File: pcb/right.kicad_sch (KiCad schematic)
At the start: 55 parts, among them SW1 SW_PUSH, SW10 SW_PUSH, SW11 SW_PUSH, SW12 SW_PUSH, SW13 SW_PUSH, SW14 SW_PUSH, SW15 SW_PUSH, SW16 SW_PUSH, SW17 SW_PUSH, SW18 SW_PUSH, SW19 SW_PUSH, SW2 SW_PUSH, SW20 SW_PUSH, SW3 SW_PUSH, SW4 SW_PUSH, SW5 SW_PUSH, SW6 SW_PUSH, SW7 SW_PUSH, SW8 SW_PUSH, SW9 SW_PUSH, U1 xiao-ble

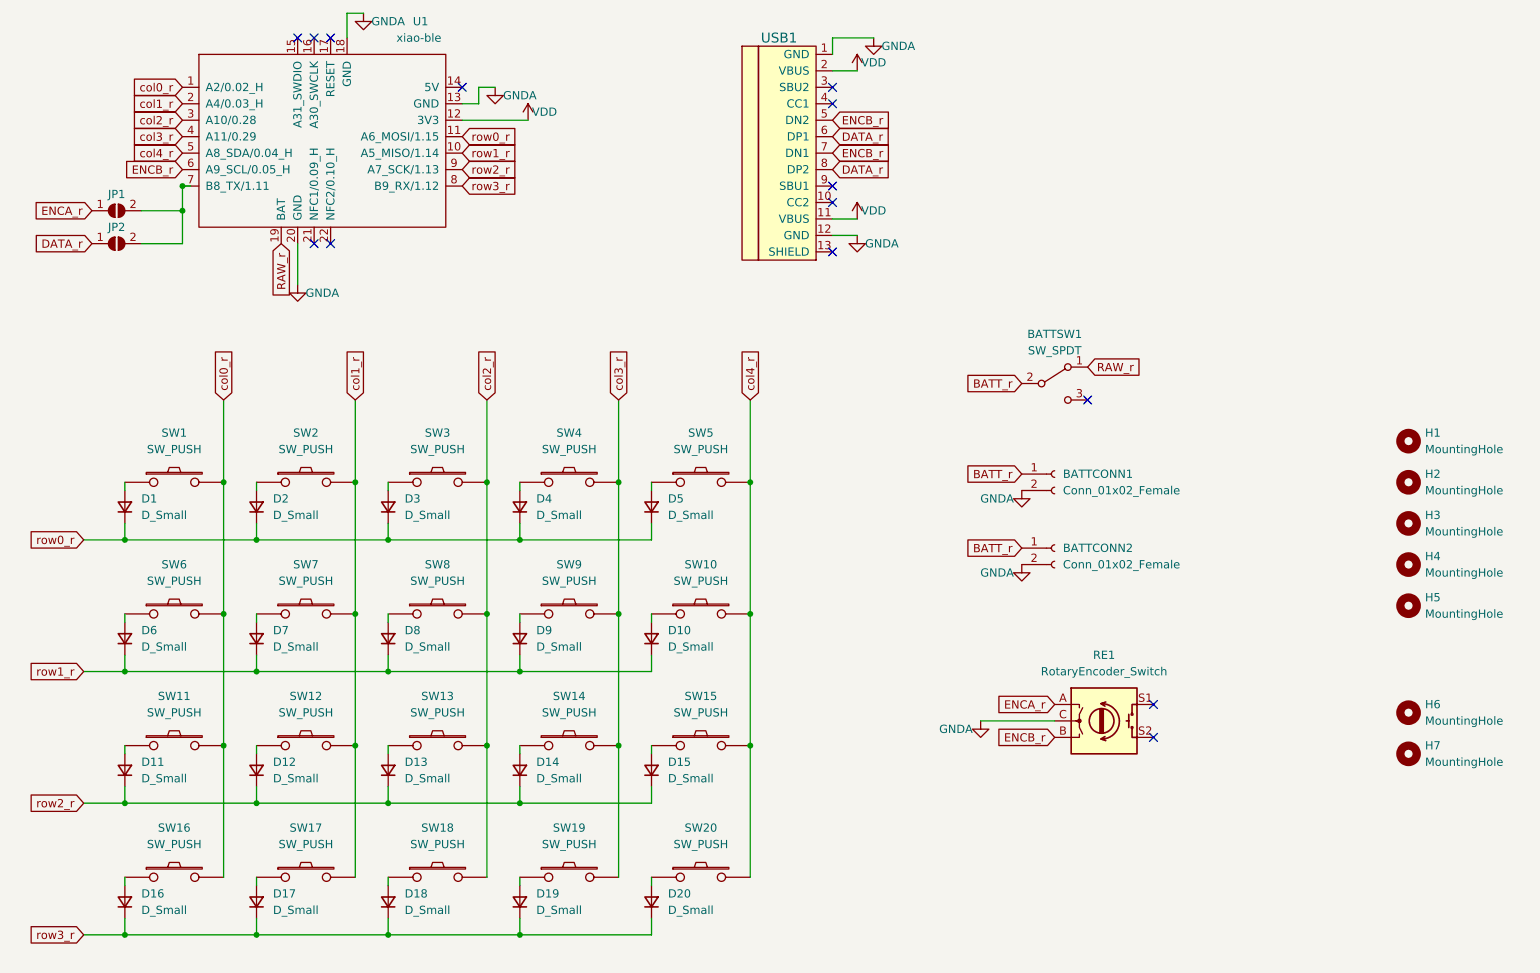
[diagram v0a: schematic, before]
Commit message: udpate pcb, remove unused files
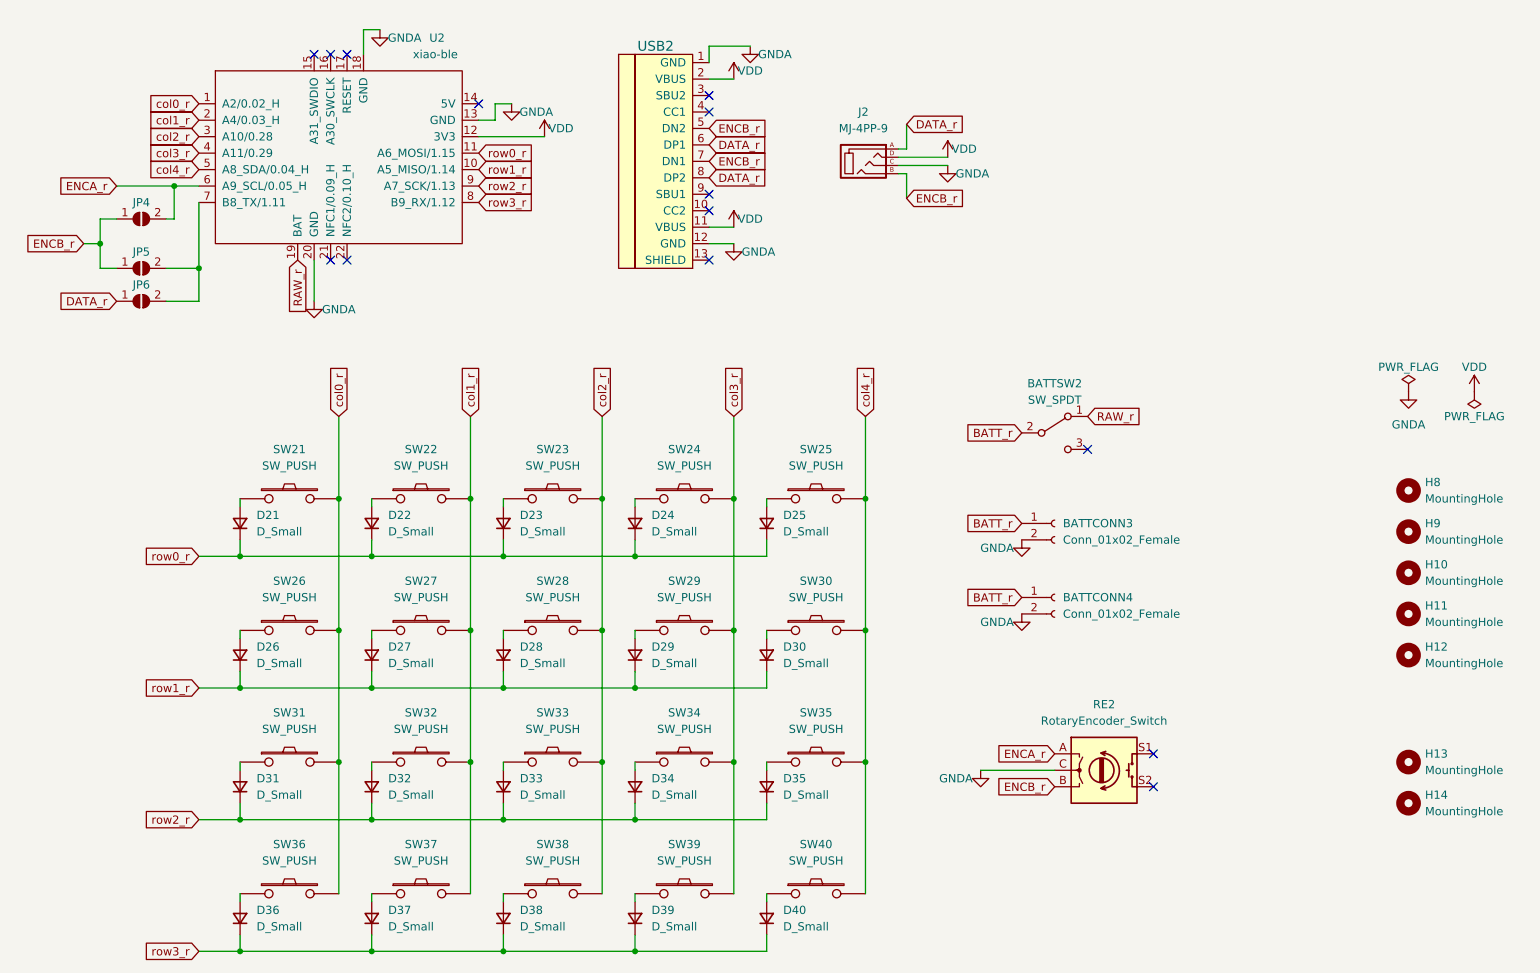
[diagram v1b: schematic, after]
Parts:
- removed BATTCONN1, BATTCONN2: Conn_01x02_Female, pica:JST_PH_S2B-PH-K_1x02_P2.00mm, symbol Connector:Conn_01x02_Female
- removed BATTSW1: SW_SPDT, Button_Switch_SMD:SW_SPDT_PCM12, symbol Switch:SW_SPDT
- removed D1, D10, D11, D12, D13, D14, D15, D16, D17, D18, D19, D2, D20, D3, D4, D5, D6, D7, D8, D9: D_Small, pica:D3_SMD, symbol Device:D_Small
- removed H1, H2, H3, H4, H5: MountingHole, pica:spacer_m2_3.4, symbol Mechanical:MountingHole
- removed H6, H7: MountingHole, kbd:thread_m2, symbol Mechanical:MountingHole
- removed JP1, JP2: SolderJumper_2_Open, Jumper:SolderJumper-2_P1.3mm_Open_TrianglePad1.0x1.5mm, symbol Jumper:SolderJumper_2_Open
- removed RE1: RotaryEncoder_Switch, pica:RotaryEncoder_EC11, symbol Device:RotaryEncoder_Switch
- removed SW1, SW10, SW11, SW12, SW13, SW14, SW15, SW16, SW17, SW18, SW19, SW2, SW3, SW4, SW5, SW6, SW7, SW8, SW9: SW_PUSH, pica:CherryMX_Hotswap_ChocV2, symbol kbd:SW_PUSH
- removed SW20: SW_PUSH, pica:CherryMX_Hotswap_ChocV2_1.5, symbol kbd:SW_PUSH
- removed U1: xiao-ble, pica:xiao-ble-tht, symbol kleeb-mcu:xiao-ble
- removed USB1: HRO-TYPE-C-31-M-12, pica:HRO-TYPE-C-31-M-12-data, symbol typec:HRO-TYPE-C-31-M-12
- added BATTCONN3, BATTCONN4: Conn_01x02_Female, pica:JST_PH_S2B-PH-K_1x02_P2.00mm, symbol Connector:Conn_01x02_Female
- added BATTSW2: SW_SPDT, Button_Switch_SMD:SW_SPDT_PCM12, symbol Switch:SW_SPDT
- added D21, D22, D23, D24, D25, D26, D27, D28, D29, D30, D31, D32, D33, D34, D35, D36, D37, D38, D39, D40: D_Small, pica:D3_SMD, symbol Device:D_Small
- added H10, H11, H12, H8, H9: MountingHole, pica:spacer_m2_3.4, symbol Mechanical:MountingHole
- added H13, H14: MountingHole, kbd:thread_m2, symbol Mechanical:MountingHole
- added J2: MJ-4PP-9, pica:MJ-4PP-9_1side, symbol kbd:MJ-4PP-9
- added JP4, JP5, JP6: SolderJumper_2_Open, Jumper:SolderJumper-2_P1.3mm_Open_TrianglePad1.0x1.5mm, symbol Jumper:SolderJumper_2_Open
- added RE2: RotaryEncoder_Switch, pica:RotaryEncoder_EC11, symbol Device:RotaryEncoder_Switch
- added SW21, SW22, SW23, SW24, SW25, SW26, SW27, SW28, SW29, SW30, SW31, SW32, SW33, SW34, SW35, SW36, SW37, SW38, SW39: SW_PUSH, pica:CherryMX_Hotswap_ChocV2, symbol kbd:SW_PUSH
- added SW40: SW_PUSH, pica:CherryMX_Hotswap_ChocV2_1.5, symbol kbd:SW_PUSH
- added U2: xiao-ble, pica:xiao-ble-tht, symbol kleeb-mcu:xiao-ble
- added USB2: HRO-TYPE-C-31-M-12, pica:HRO-TYPE-C-31-M-12-data, symbol typec:HRO-TYPE-C-31-M-12
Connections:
- net BATT_r: now also BATTCONN3.1 (Pin_1), BATTCONN4.1 (Pin_1), BATTSW2.2 (B)
- net DATA_r: now also J2.A, JP6.1 (A), USB2.6 (DP1), USB2.8 (DP2)
- net ENCA_r: now also JP4.2 (B), RE2.A, U2.6 (A9_SCL/0.05_H)
- net ENCB_r: now also J2.B, JP4.1 (A), JP5.1 (A), RE2.B, USB2.5 (DN2), USB2.7 (DN1)
- net GNDA: now also BATTCONN3.2 (Pin_2), BATTCONN4.2 (Pin_2), J2.C, RE2.C, U2.13 (GND), U2.18 (GND), U2.20 (GND), USB2.1 (GND), USB2.12 (GND)
- net RAW_r: now also BATTSW2.1 (A), U2.19 (BAT)
- net VDD: now also J2.D, U2.12 (3V3), USB2.11 (VBUS), USB2.2 (VBUS)
- net col0_r: now also SW21.2, SW26.2, SW31.2, SW36.2, U2.1 (A2/0.02_H)
- net col1_r: now also SW22.2, SW27.2, SW32.2, SW37.2, U2.2 (A4/0.03_H)
- net col2_r: now also SW23.2, SW28.2, SW33.2, SW38.2, U2.3 (A10/0.28)
- net col3_r: now also SW24.2, SW29.2, SW34.2, SW39.2, U2.4 (A11/0.29)
- net col4_r: now also SW25.2, SW30.2, SW35.2, SW40.2, U2.5 (A8_SDA/0.04_H)
- net row0_r: now also D21.1 (K), D22.1 (K), D23.1 (K), D24.1 (K), D25.1 (K), U2.11 (A6_MOSI/1.15)
- net row1_r: now also D26.1 (K), D27.1 (K), D28.1 (K), D29.1 (K), D30.1 (K), U2.10 (A5_MISO/1.14)
- net row2_r: now also D31.1 (K), D32.1 (K), D33.1 (K), D34.1 (K), D35.1 (K), U2.9 (A7_SCK/1.13)
- net row3_r: now also D36.1 (K), D37.1 (K), D38.1 (K), D39.1 (K), D40.1 (K), U2.8 (B9_RX/1.12)
- new net: D26.2 (A), SW26.1
- new net: D24.2 (A), SW24.1
- new net: D27.2 (A), SW27.1
- new net: JP5.2 (B), JP6.2 (B), U2.7 (B8_TX/1.11)
- new net: D30.2 (A), SW30.1
- new net: D35.2 (A), SW35.1
- new net: D28.2 (A), SW28.1
- new net: D37.2 (A), SW37.1
- new net: D29.2 (A), SW29.1
- new net: D33.2 (A), SW33.1
- new net: D23.2 (A), SW23.1
- new net: D32.2 (A), SW32.1
- new net: D36.2 (A), SW36.1
- new net: D22.2 (A), SW22.1
- new net: D34.2 (A), SW34.1
- new net: D40.2 (A), SW40.1
- new net: D21.2 (A), SW21.1
- new net: D38.2 (A), SW38.1
- new net: D25.2 (A), SW25.1
- new net: D39.2 (A), SW39.1
- new net: D31.2 (A), SW31.1
